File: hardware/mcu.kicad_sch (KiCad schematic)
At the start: 30 parts, among them Q1 MMBT3904, Q2 MMBT3904, U1 ESP32-C3, Y1 40MHz

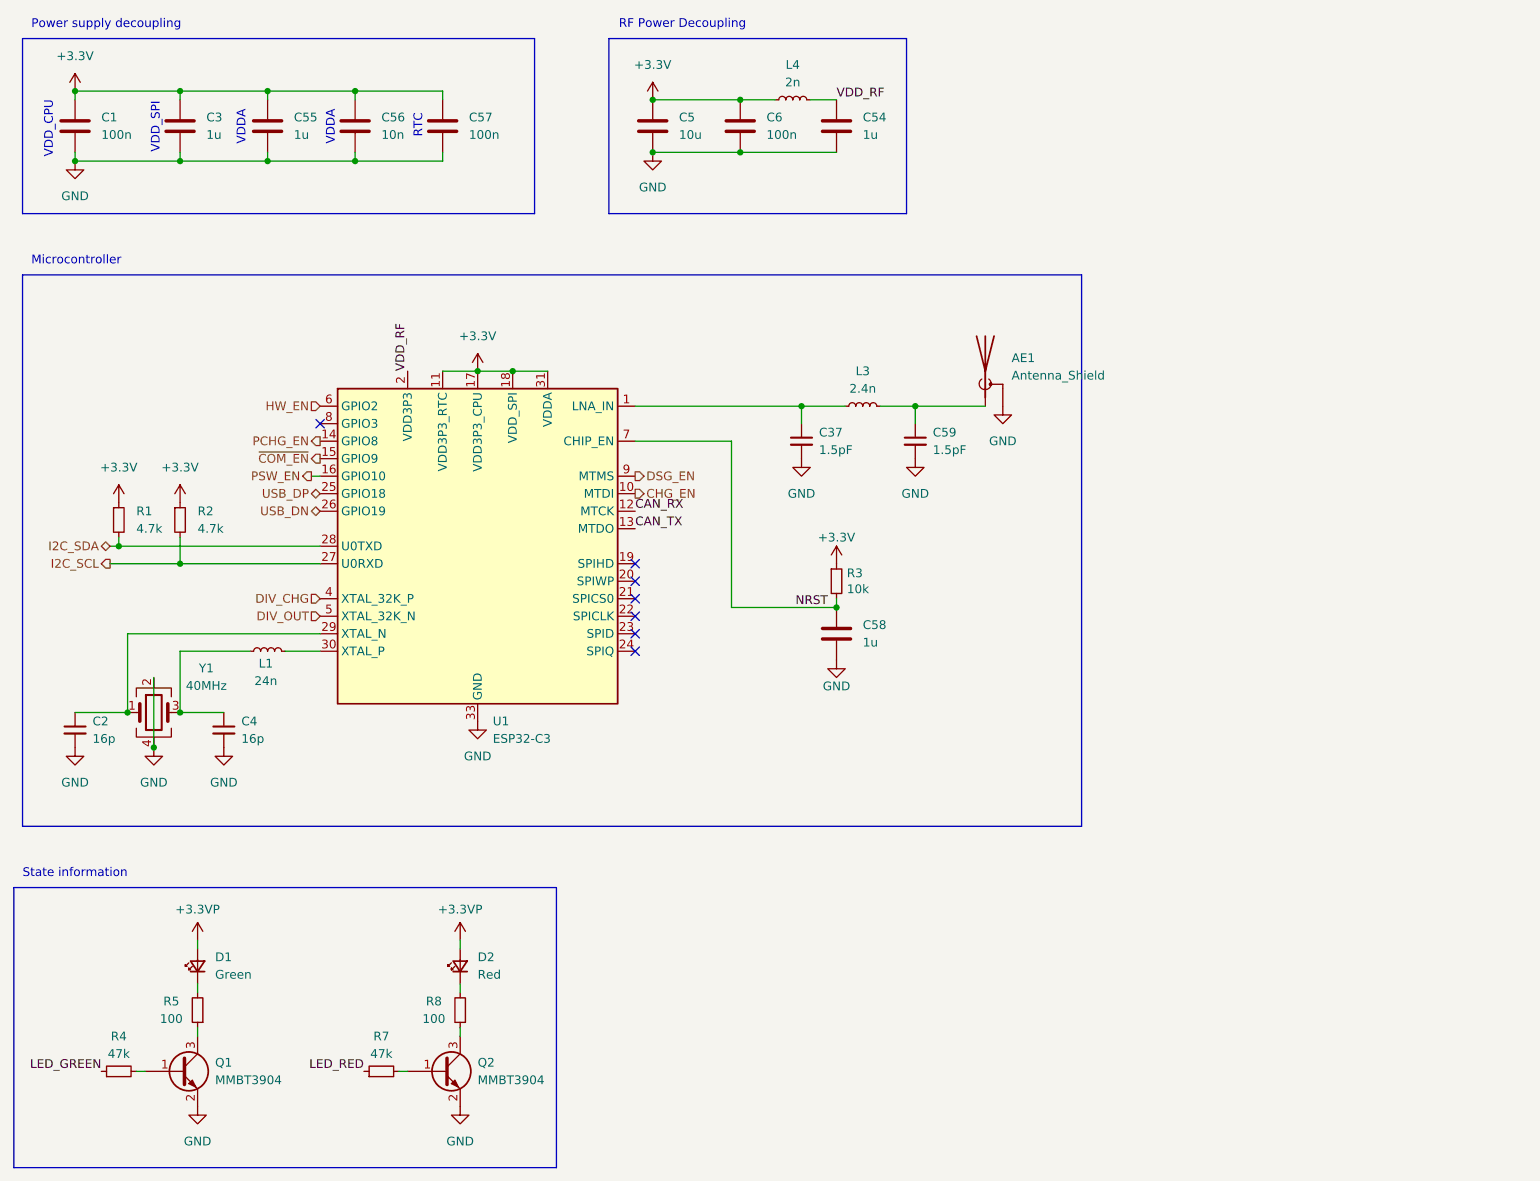
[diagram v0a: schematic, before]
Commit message: MCU circuit sourced complete
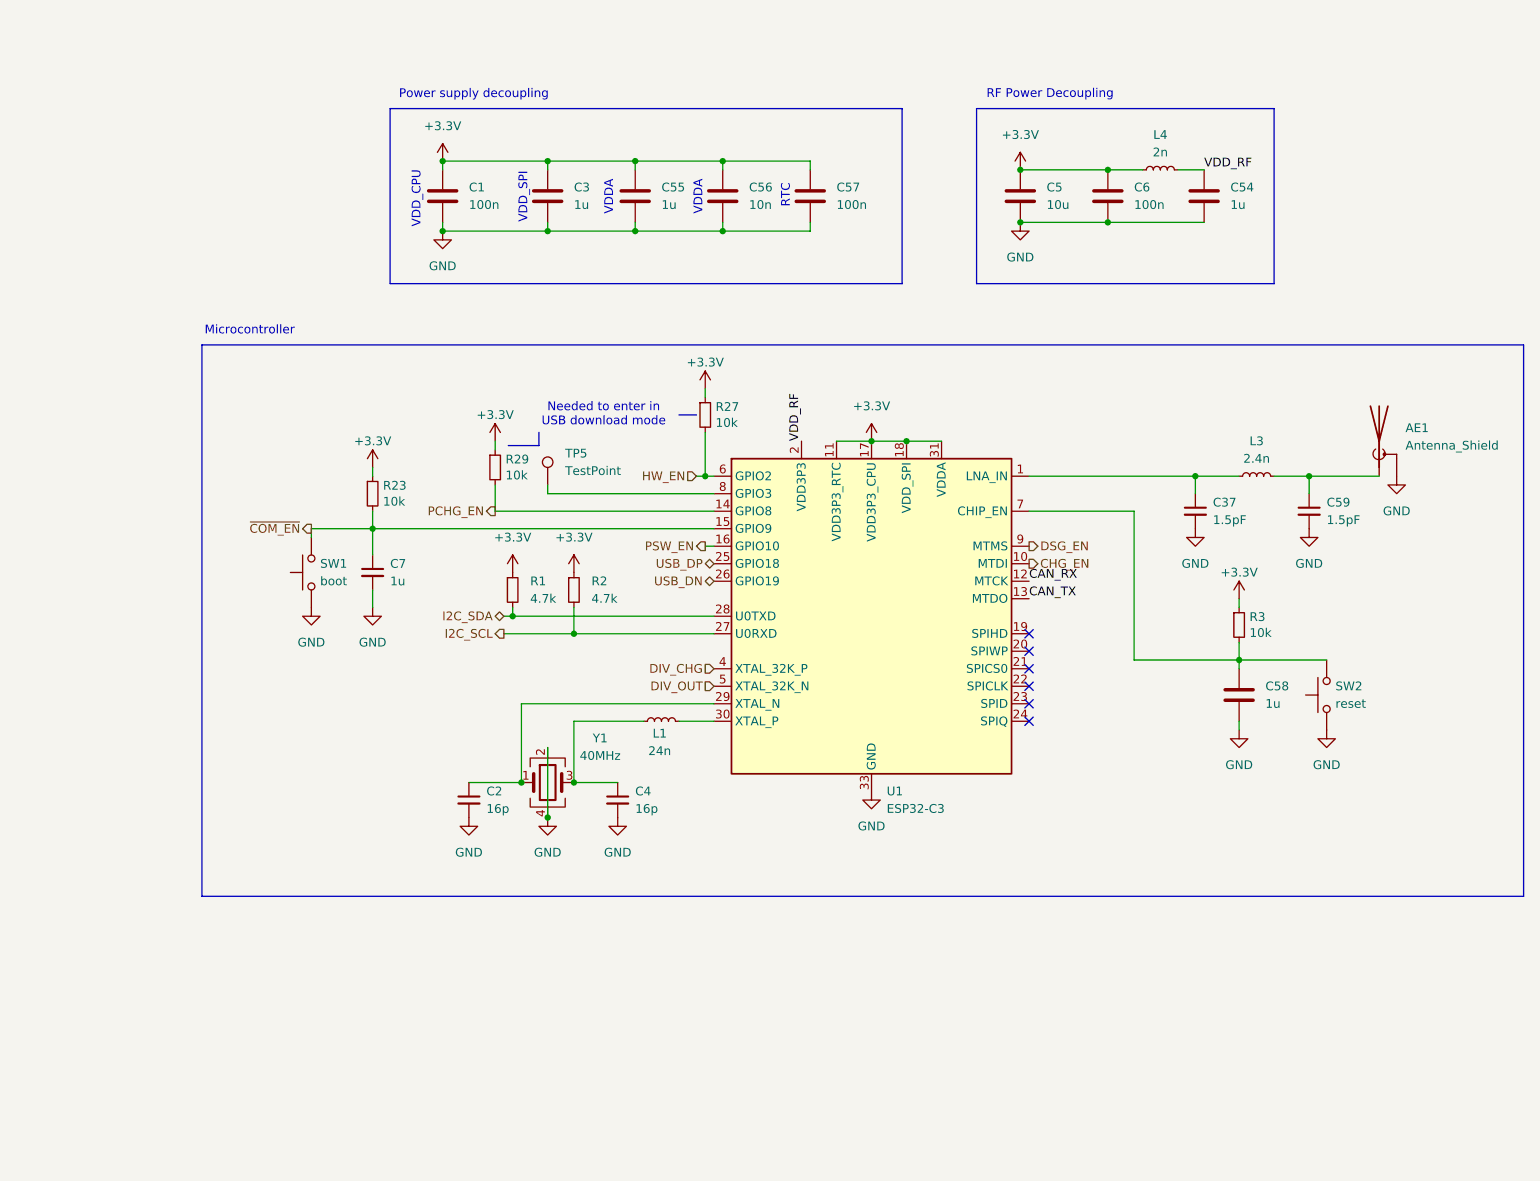
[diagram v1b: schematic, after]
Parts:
- removed D1: Green, LED_SMD:LED_0805_2012Metric, symbol Device:LED_Small
- removed D2: Red, LED_SMD:LED_0805_2012Metric, symbol Device:LED_Small
- removed Q1, Q2: MMBT3904, Package_TO_SOT_SMD:SOT-23, symbol Transistor_BJT:MMBT3904
- removed R4, R7: 47k, Resistor_SMD:R_0402_1005Metric, symbol Device:R_Small
- removed R5, R8: 100, Resistor_SMD:R_0603_1608Metric, symbol Device:R_Small
- added C7: 1u, Capacitor_SMD:C_0402_1005Metric, symbol Device:C_Small
- added R23, R27, R29: 10k, Resistor_SMD:R_0603_1608Metric, symbol Device:R_Small
- added SW1: boot, Button_Switch_SMD:SW_Push_SPST_NO_Alps_SKRK, symbol Switch:SW_Push
- added SW2: reset, Button_Switch_SMD:SW_Push_SPST_NO_Alps_SKRK, symbol Switch:SW_Push
- added TP5: TestPoint, symbol Connector:TestPoint
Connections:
- net +3.3V: now also R23.1, R27.1, R29.1
- net GND: now also C7.2, SW1.1, SW2.1
- net HW_EN: now also R27.2
- net PCHG_EN: now also R29.2
- net ~{COM_EN}: now also C7.1, R23.2, SW1.2
- net at U1.8 (GPIO3): now also TP5.1
- net NRST: no longer names the net of C58.1, R3.2, U1.7 (CHIP_EN)
- net NRST: now also SW2.2
- no-connect marks 7 -> 6
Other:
- note added: "Needed to enter in USB download mode"
- note removed: "State information"
- moved on the sheet: AE1, C1, C2, C3, C37, C4, C5, C54, C55, C56, C57, C58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

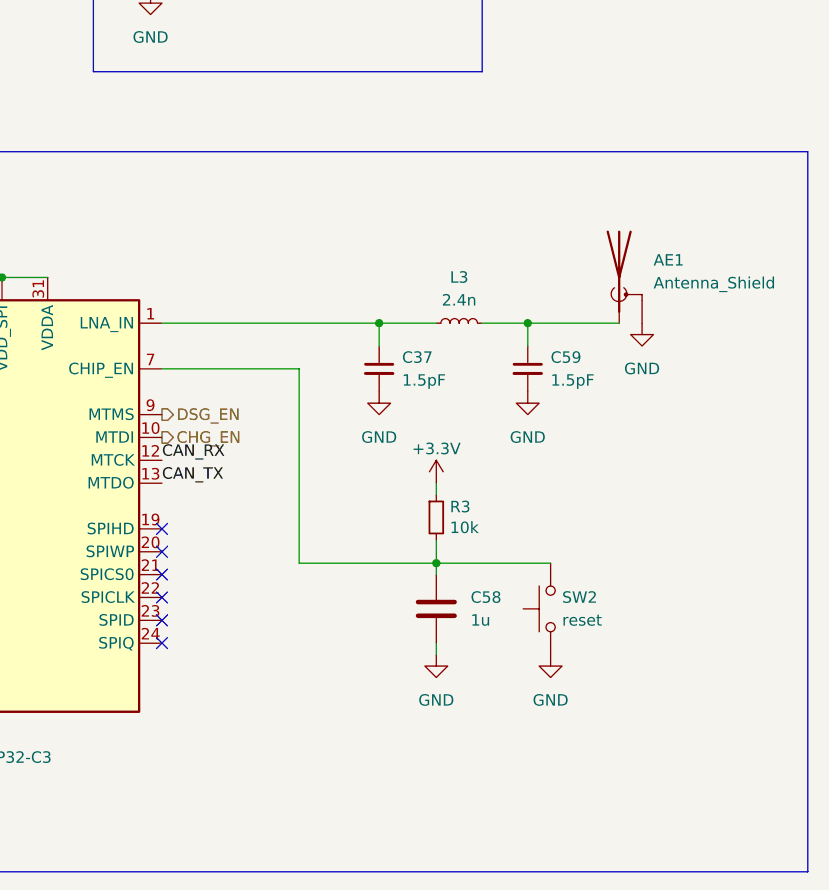
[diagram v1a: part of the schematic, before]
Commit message: Thermistor conenctions
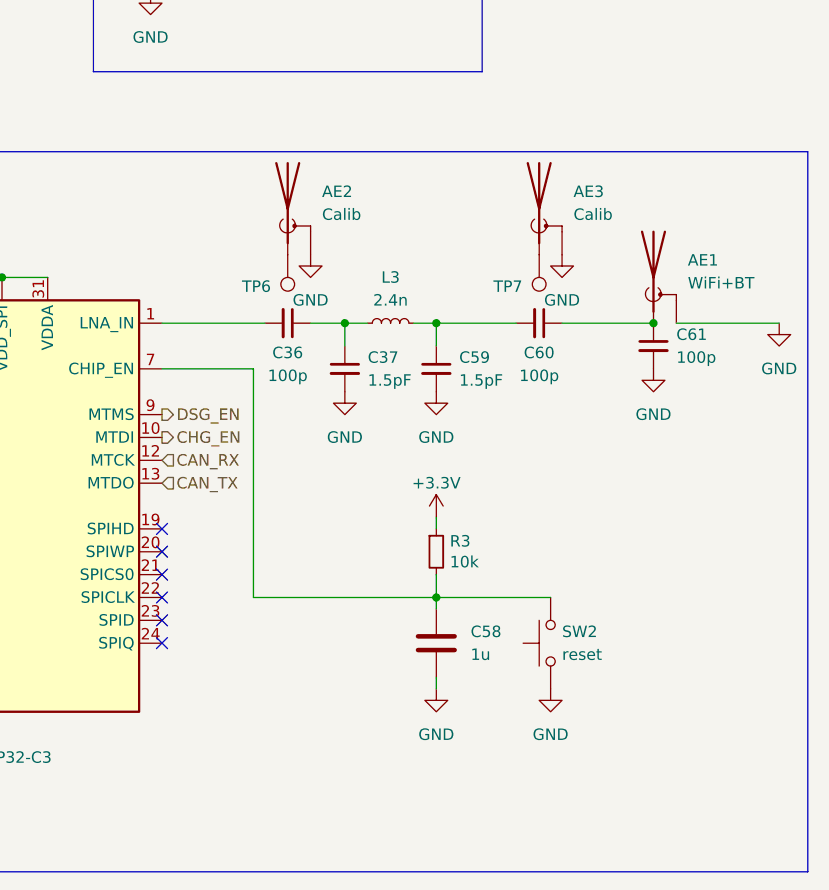
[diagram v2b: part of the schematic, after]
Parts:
- added AE2, AE3: Calib, Connector_Coaxial:U.FL_Hirose_U.FL-R-SMT-1_Vertical, symbol Device:Antenna_Shield
- added C36, C60: 100p, Capacitor_SMD:C_0402_1005Metric, symbol Device:C_Small
- added C61: 100p, symbol Device:C_Small
- added TP6, TP7: TestPoint, Capacitor_SMD:C_0402_1005Metric, symbol Connector:TestPoint
- AE1: value Antenna_Shield -> WiFi+BT
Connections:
- net GND: now also AE2.2 (Shield), AE3.2 (Shield), C61.2
- net at C37.1, L3.1: now also C36.1; no longer U1.1 (LNA_IN)
- net at C59.1, L3.2: now also C60.2; no longer AE1.1 (A)
- new net: AE3.1 (A), TP7.1
- new net: C36.2, U1.1 (LNA_IN)
- new net: AE1.1 (A), C60.1, C61.1
- new net: AE2.1 (A), TP6.1
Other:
- moved on the sheet: AE1, C37, C58, C59, L3, R3, SW2
